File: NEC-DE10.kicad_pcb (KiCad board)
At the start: 2 copper layers, 110.5 x 72.4 mm, 12 parts, among them U3 74ALVC164245, U4 74ALVC164245, U5 74ALVC164245

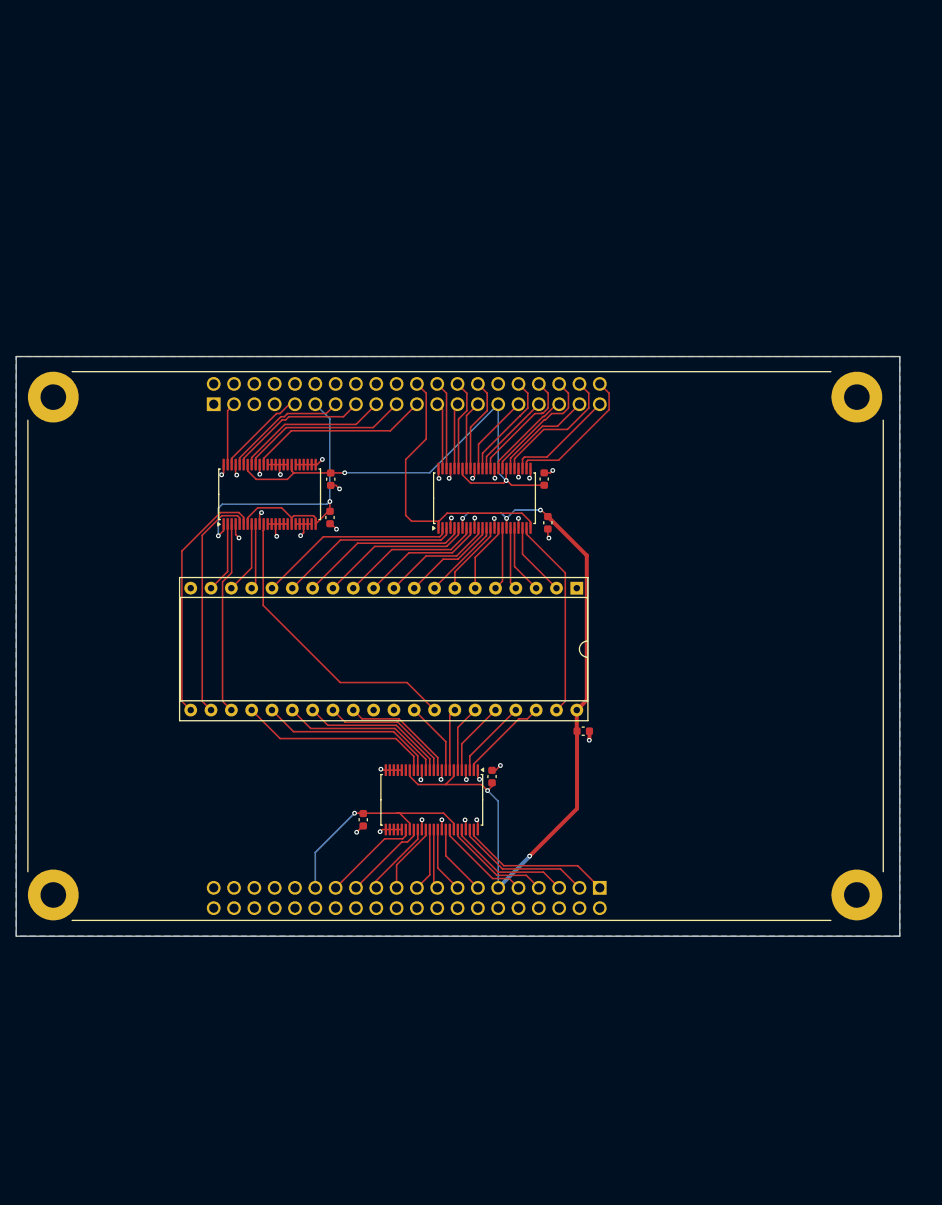
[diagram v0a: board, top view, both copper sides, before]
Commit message: Added V35 board
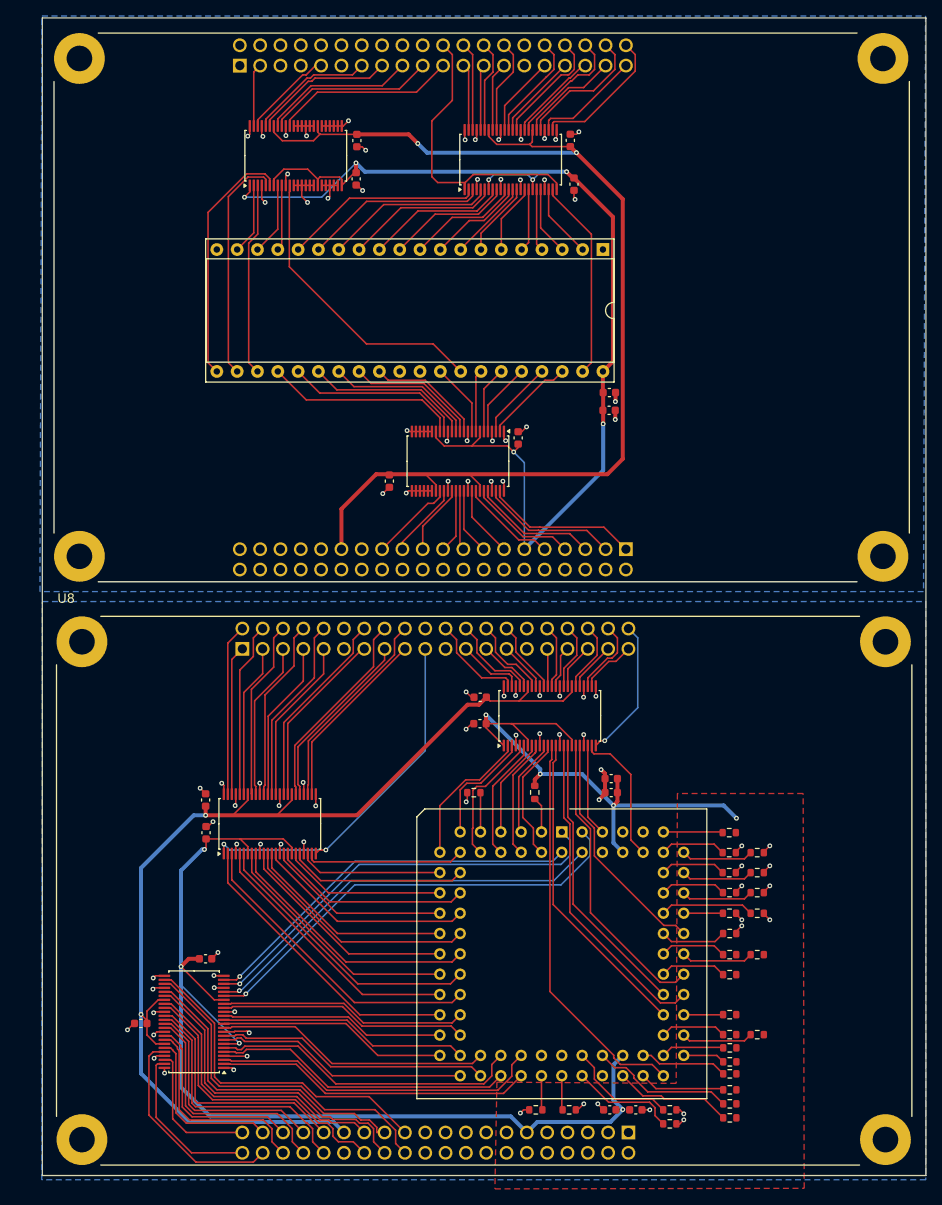
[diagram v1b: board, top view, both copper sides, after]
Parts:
- added C10: 100nF, Capacitor_SMD:C_0603_1608Metric, F.Cu at (116.7, 113.0)
- added C11: 100nF, Capacitor_SMD:C_0603_1608Metric, F.Cu at (151.0, 103.5)
- added C12: 100nF, Capacitor_SMD:C_0603_1608Metric, F.Cu at (108.6, 140.9)
- added C13: 100nF, Capacitor_SMD:C_0603_1608Metric, F.Cu at (116.7, 132.9)
- added C14: 100nF, Capacitor_SMD:C_0603_1608Metric, F.Cu at (170.5, 151.8)
- added C15: 100nF, Capacitor_SMD:C_0603_1608Metric, F.Cu at (167.4, 112.1)
- added C16: 1uF, Capacitor_SMD:C_0603_1608Metric, F.Cu at (167.4, 110.3)
- added C17: 1uF, Capacitor_SMD:C_0603_1608Metric, F.Cu at (167.2, 151.8)
- added C18: 1uF, Capacitor_SMD:C_0603_1608Metric, F.Cu at (167.2, 64.3)
- added C8: 100nF, Capacitor_SMD:C_0603_1608Metric, F.Cu at (151.1, 100.2)
- added C9: 100nF, Capacitor_SMD:C_0603_1608Metric, F.Cu at (116.8, 117.1)
- added R1: 10k, Resistor_SMD:R_0603_1608Metric, F.Cu at (182.2, 129.7)
- added R10: 10k, Resistor_SMD:R_0603_1608Metric, F.Cu at (182.2, 149.2)
- added R11: 10k, Resistor_SMD:R_0603_1608Metric, F.Cu at (182.2, 147.2)
- added R12: 10k, Resistor_SMD:R_0603_1608Metric, F.Cu at (182.2, 145.8)
- added R13: 10k, Resistor_SMD:R_0603_1608Metric, F.Cu at (182.2, 144.0)
- added R14: 10k, Resistor_SMD:R_0603_1608Metric, F.Cu at (185.7, 142.3)
- added R15: 10k, Resistor_SMD:R_0603_1608Metric, F.Cu at (182.2, 142.3)
- added R16: 10k, Resistor_SMD:R_0603_1608Metric, F.Cu at (182.2, 139.8)
- added R17: 10k, Resistor_SMD:R_0603_1608Metric, F.Cu at (182.2, 134.8)
- added R18: 10k, Resistor_SMD:R_0603_1608Metric, F.Cu at (185.7, 132.3)
- added R19: 10k, Resistor_SMD:R_0603_1608Metric, F.Cu at (182.2, 132.3)
- added R2: 10k, Resistor_SMD:R_0603_1608Metric, F.Cu at (182.2, 127.2)
- added R20: 10k, Resistor_SMD:R_0603_1608Metric, F.Cu at (158.0, 151.8)
- added R21: 10k, Resistor_SMD:R_0603_1608Metric, F.Cu at (162.2, 151.8)
- added R22: 10k, Resistor_SMD:R_0603_1608Metric, F.Cu at (174.8, 153.5)
- added R23: 10k, Resistor_SMD:R_0603_1608Metric, F.Cu at (174.8, 151.8)
- added R24: 10k, Resistor_SMD:R_0603_1608Metric, F.Cu at (182.2, 119.6)
- added R25: 10k, Resistor_SMD:R_0603_1608Metric, F.Cu at (157.9, 112.1)
- added R26: 10k, Resistor_SMD:R_0603_1608Metric, F.Cu at (182.2, 152.8)
- added R27: 10k, Resistor_SMD:R_0603_1608Metric, F.Cu at (182.2, 117.1)
- added R28: 10k, Resistor_SMD:R_0603_1608Metric, F.Cu at (150.3, 112.1)
- added R3: 10k, Resistor_SMD:R_0603_1608Metric, F.Cu at (185.7, 127.2)
- added R4: 10k, Resistor_SMD:R_0603_1608Metric, F.Cu at (185.7, 124.6)
- added R5: 10k, Resistor_SMD:R_0603_1608Metric, F.Cu at (182.2, 124.6)
- added R6: 10k, Resistor_SMD:R_0603_1608Metric, F.Cu at (185.7, 122.1)
- added R7: 10k, Resistor_SMD:R_0603_1608Metric, F.Cu at (182.2, 122.1)
- added R8: 10k, Resistor_SMD:R_0603_1608Metric, F.Cu at (185.7, 119.6)
- added R9: 10k, Resistor_SMD:R_0603_1608Metric, F.Cu at (182.2, 151.0)
- added U10: 74ALVC164245, Package_SO:TSSOP-48_6.1x12.5mm_P0.5mm, F.Cu at (159.8, 102.5)
- added U6: 74ALVC164245, Package_SO:TSSOP-48_6.1x12.5mm_P0.5mm, F.Cu at (115.3, 140.8)
- added U7: 74ALVC164245, Package_SO:TSSOP-48_6.1x12.5mm_P0.5mm, F.Cu at (124.8, 116.0)
- added U8: ~, NEC-DE10:MODULE_P0496, F.Cu at (101.3, 155.5)
- added U9: ~, Package_LCC:PLCC-84_THT-Socket, F.Cu at (161.2, 117.0)
- moved C1 42.5 mm to (162.3, 30.6)
- moved C4 42.5 mm to (162.8, 36.0)
- moved U1 42.5 mm to (166.4, 44.2)
- moved U5 42.5 mm to (128.0, 32.5)
- moved C2 42.5 mm to (135.6, 30.6)
- moved C3 42.5 mm to (139.7, 73.2)
- moved C5 42.5 mm to (155.8, 67.8)
- moved C7 42.5 mm to (167.2, 62.1)
- moved U2 42.5 mm to (101.0, 82.6)
- moved U3 42.5 mm to (154.9, 33.0)
- moved U4 42.5 mm to (148.3, 70.7)
- moved C6 42.5 mm to (135.5, 35.4)
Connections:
- net /A16 renamed /V30/A16
- net /A17 renamed /V30/A17
- net /A18 renamed /V30/A18
- net /A19 renamed /V30/A19
- net /AD0 renamed /V30/AD0
- net /AD1 renamed /V30/AD1
- net /AD10 renamed /V30/AD10
- net /AD11 renamed /V30/AD11
- net /AD12 renamed /V30/AD12
- net /AD13 renamed /V30/AD13
- net /AD14 renamed /V30/AD14
- net /AD15 renamed /V30/AD15
- net /AD2 renamed /V30/AD2
- net /AD3 renamed /V30/AD3
- net /AD4 renamed /V30/AD4
- net /AD5 renamed /V30/AD5
- net /AD6 renamed /V30/AD6
- net /AD7 renamed /V30/AD7
- net /AD8 renamed /V30/AD8
- net /AD9 renamed /V30/AD9
- net /ASTB renamed /V30/ASTB
- net /BUF~{R}/W renamed /V30/BUF~{R}/W
- net /CLK renamed /V30/CLK
- net /F_A16 renamed /V30/F_A16
- net /F_A17 renamed /V30/F_A17
- net /F_A18 renamed /V30/F_A18
- net /F_A19 renamed /V30/F_A19
- net /F_AD0 renamed /V30/F_AD0
- net /F_AD1 renamed /V30/F_AD1
- net /F_AD10 renamed /V30/F_AD10
- net /F_AD11 renamed /V30/F_AD11
- net /F_AD12 renamed /V30/F_AD12
- net /F_AD13 renamed /V30/F_AD13
- net /F_AD14 renamed /V30/F_AD14
- net /F_AD15 renamed /V30/F_AD15
- net /F_AD2 renamed /V30/F_AD2
- net /F_AD3 renamed /V30/F_AD3
- net /F_AD4 renamed /V30/F_AD4
- net /F_AD5 renamed /V30/F_AD5
- net /F_AD6 renamed /V30/F_AD6
- net /F_AD7 renamed /V30/F_AD7
- net /F_AD8 renamed /V30/F_AD8
- net /F_AD9 renamed /V30/F_AD9
- net /F_AD_DIR renamed /V30/F_AD_DIR
- net /F_ASTB renamed /V30/F_ASTB
- net /F_BUF~{R}/W renamed /V30/F_BUF~{R}/W
- net /F_CLK renamed /V30/F_CLK
- net /F_INT renamed /V30/F_INT
- net /F_NMI renamed /V30/F_NMI
- net /F_READY renamed /V30/F_READY
- net /F_RESET renamed /V30/F_RESET
- net /F_S/~{LG} renamed /V30/F_S/~{LG}
- net /F_~{BUFEN} renamed /V30/F_~{BUFEN}
- net /F_~{INTAK} renamed /V30/F_~{INTAK}
- net /F_~{IO}/M renamed /V30/F_~{IO}/M
- net /F_~{POLL} renamed /V30/F_~{POLL}
- net /F_~{RD} renamed /V30/F_~{RD}
- net /F_~{UBE} renamed /V30/F_~{UBE}
- net /F_~{WR} renamed /V30/F_~{WR}
- net /INT renamed /V30/INT
- net /NMI renamed /V30/NMI
- net /READY renamed /V30/READY
- net /RESET renamed /V30/RESET
- net /S/~{LG} renamed /V30/S/~{LG}
- net /~{BUFEN} renamed /V30/~{BUFEN}
- net /~{INTAK} renamed /V30/~{INTAK}
- net /~{IO}/M renamed /V30/~{IO}/M
- net /~{POLL} renamed /V30/~{POLL}
- net /~{RD} renamed /V30/~{RD}
- net /~{UBE} renamed /V30/~{UBE}
- net /~{WR} renamed /V30/~{WR}
- U2 pad JP1_11: +5V -> unconnected-(U2A-5V_JP1-PadJP1_11)
- U2 pad JP1_29: +3.3V -> unconnected-(U2A-3.3V_JP1-PadJP1_29)
- U2 pad JP7_27: /F_HLDAK -> unconnected-(U2C-GPIO1_24-PadJP7_27)
- U4 pad 19: /HLDAK -> GND
- U4 pad 30: /F_HLDAK -> GND
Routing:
- net +5V: track 142.8 -> 358.3 mm, vias 7 -> 15
- net +3.3V: track 88.8 -> 294.4 mm, vias 3 -> 4
- net GND: track 58.5 -> 138.1 mm, vias 36 -> 93
- net /V35/R/~{W}: track 0.00 -> 56.4 mm, vias 0 -> 1
- net /V35/~{IOSTB}: track 0.00 -> 53.3 mm, vias 0 -> 1
- net /V35/~{MSTB}: track 0.00 -> 52.0 mm, vias 0 -> 1
- net /V35/N/~{S}: track 0.00 -> 49.6 mm
- net /V35/~{MREQ}: track 0.00 -> 48.9 mm, vias 0 -> 1
- net /V35/F_D_DIR: track 0.00 -> 46.0 mm, vias 0 -> 2
- net /V35/F_~{IOSTB}: track 0.00 -> 43.7 mm
- net /V35/F_~{MREQ}: track 0.00 -> 41.9 mm
- net /V35/A11: track 0.00 -> 41.4 mm
- net /V35/~{INTP0}: track 0.00 -> 40.5 mm
- net /V35/F_R/~{W}: track 0.00 -> 40.5 mm
- net /V35/A10: track 0.00 -> 39.6 mm
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- added copper zone on F.Cu, net +5V
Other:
- board size 110.5 x 72.4 mm -> 110.4 x 144.7 mm
